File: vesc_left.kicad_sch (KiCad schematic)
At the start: 21 parts, among them J2 HALL_ENC, J6 USB, SW1 SENS_VOLTAGE

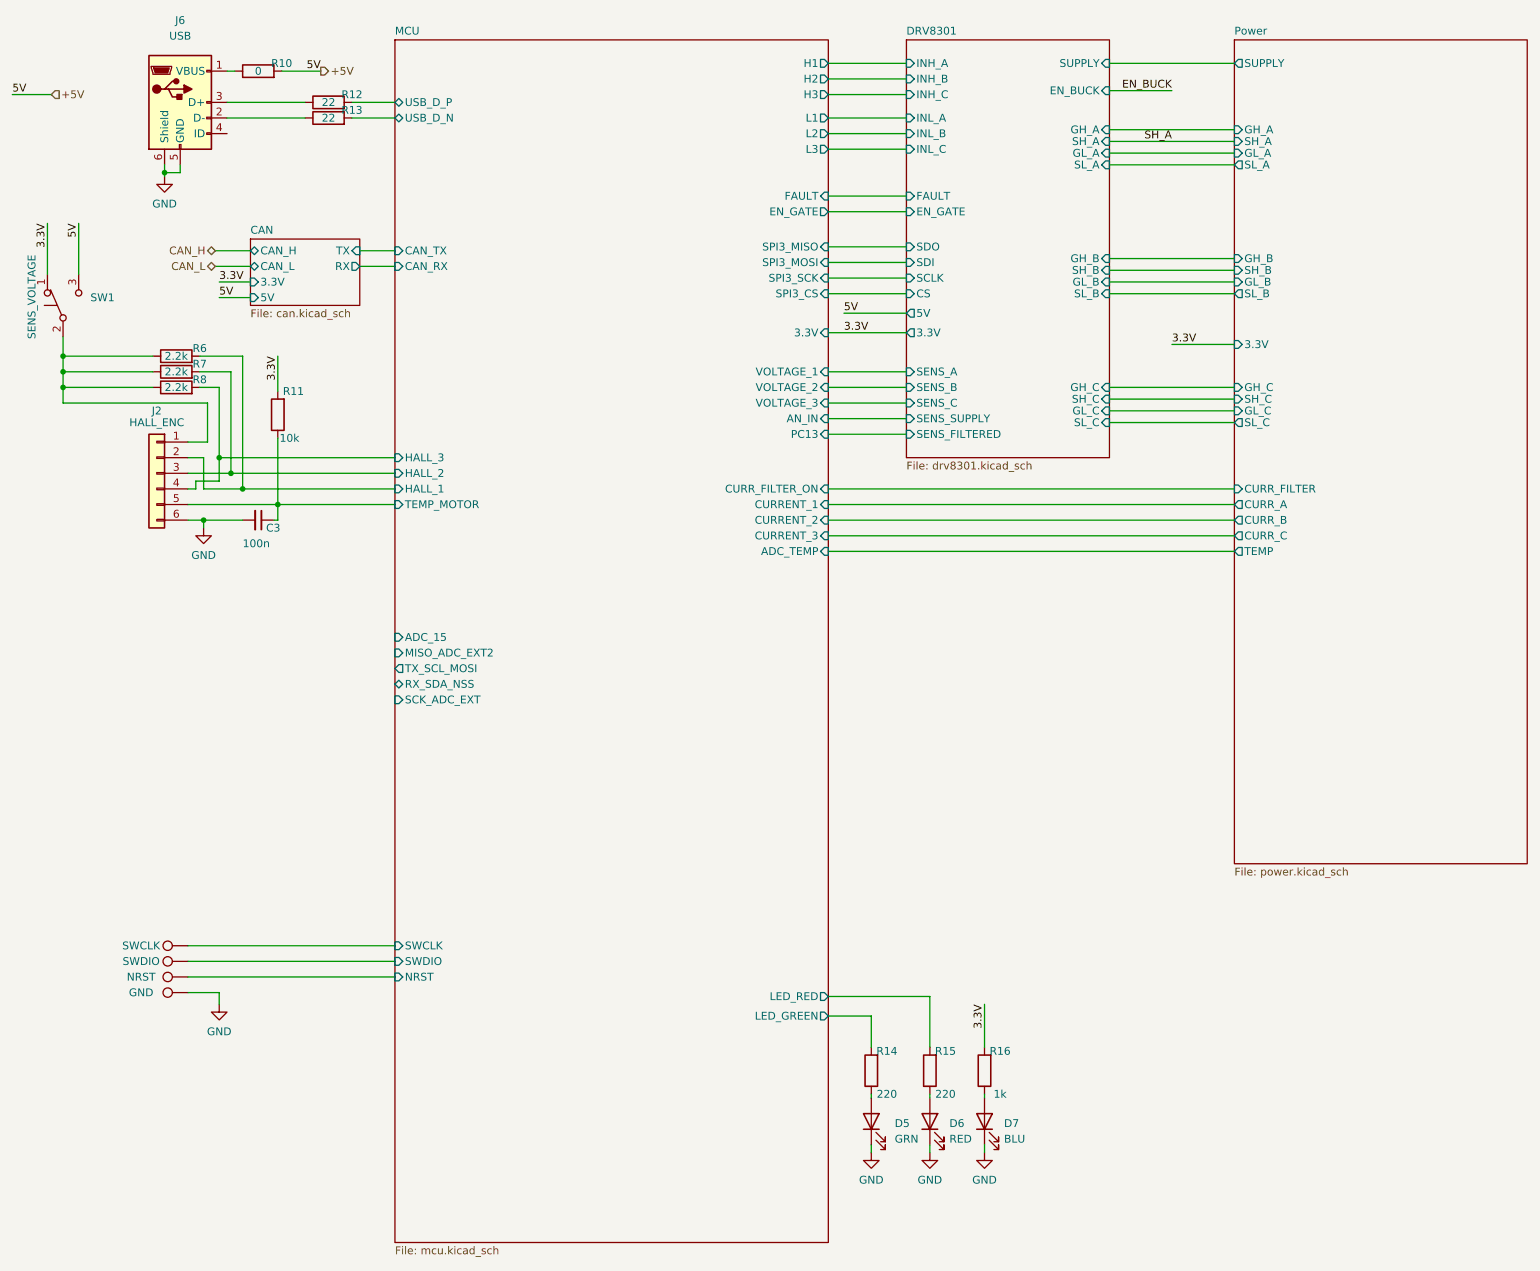
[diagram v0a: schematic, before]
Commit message: Update
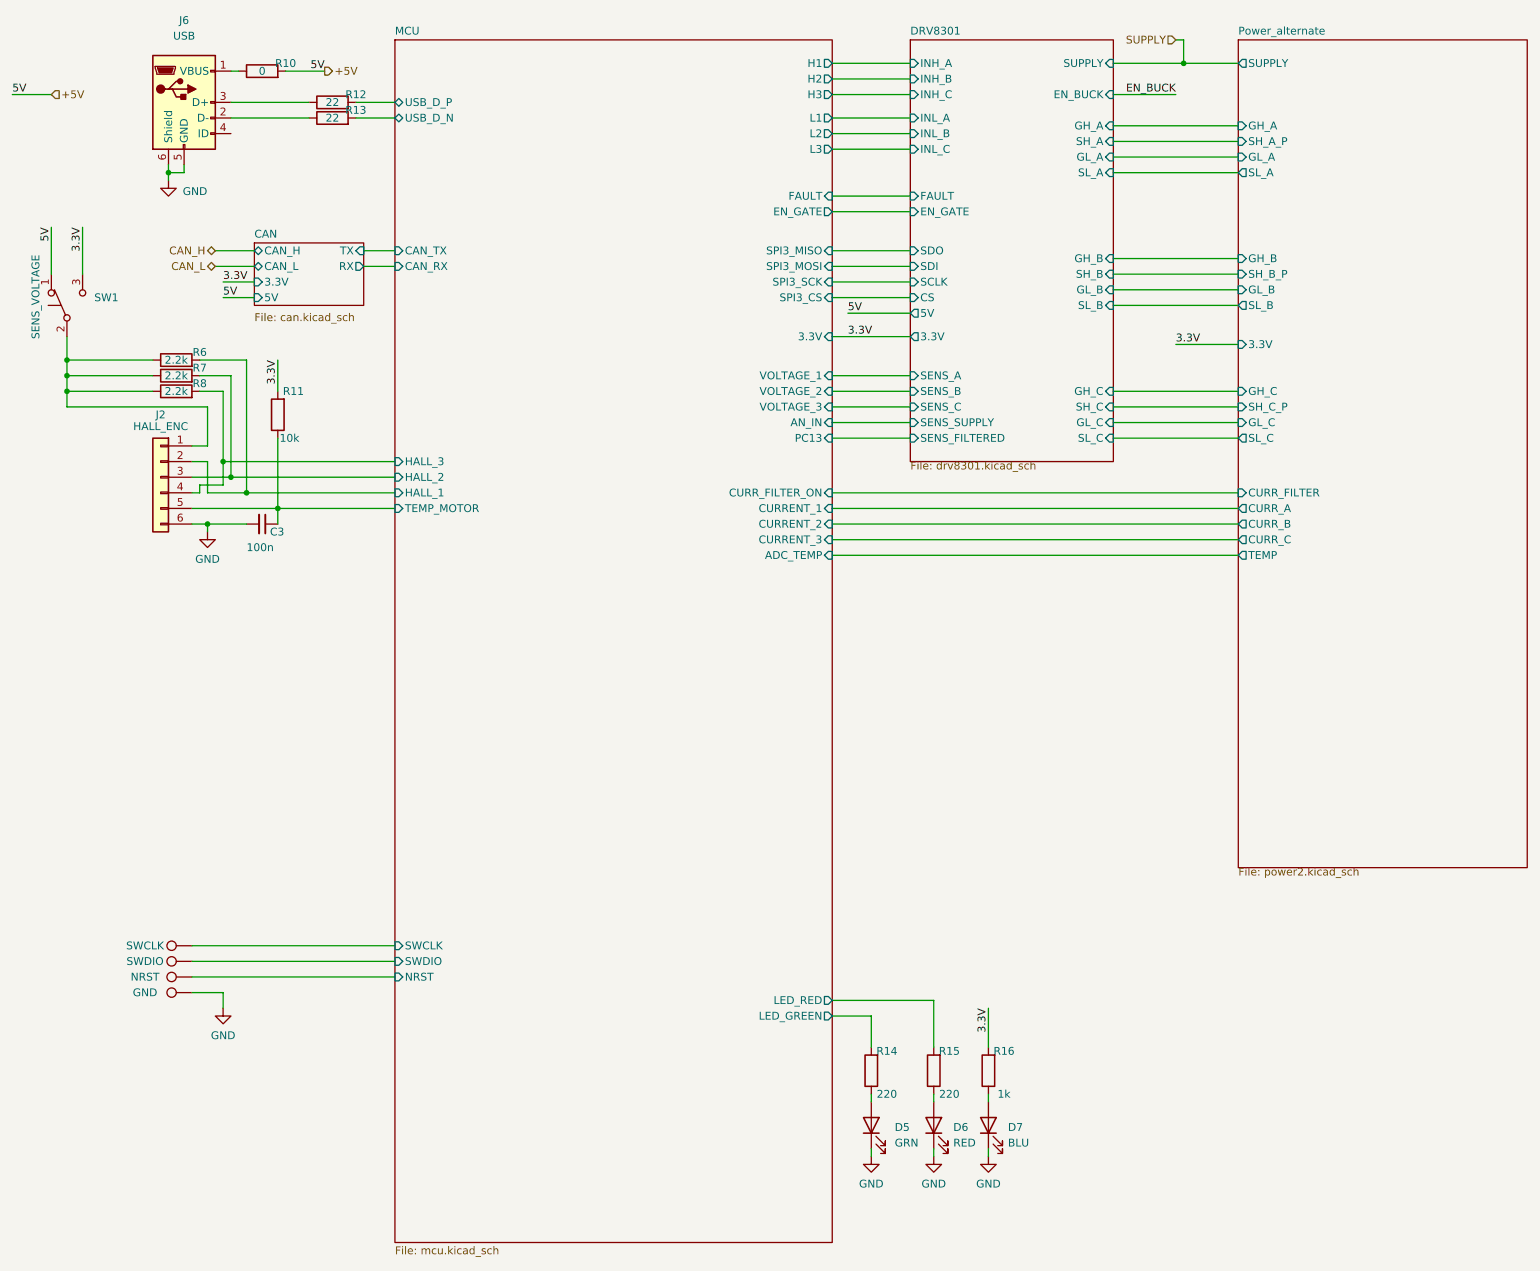
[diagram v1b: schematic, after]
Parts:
- C3: Voltage 50V -> 100V
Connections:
- net +5V: now also SW1.1 (A); no longer SW1.3 (C)
- net 3.3V: now also SW1.3 (C); no longer SW1.1 (A)
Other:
- sheet Power renamed Power_alternate
- sheet MCU ports: added none; removed ADC_15, MISO_ADC_EXT2, RX_SDA_NSS, SCK_ADC_EXT, TX_SCL_MOSI
- sheet Power_alternate: file power.kicad_sch -> power2.kicad_sch
- sheet Power_alternate ports: added SH_A_P, SH_B_P, SH_C_P; removed SH_A, SH_B, SH_C
- moved on the sheet: C3, D5, D6, D7, J2, J6, R10, R12, R13, R15, R16, R6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
